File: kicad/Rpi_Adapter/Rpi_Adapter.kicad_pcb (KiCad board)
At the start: 2 copper layers, 65 x 22 mm, 49 parts, among them P1 CONN_02X20, P2 CONN_02X03

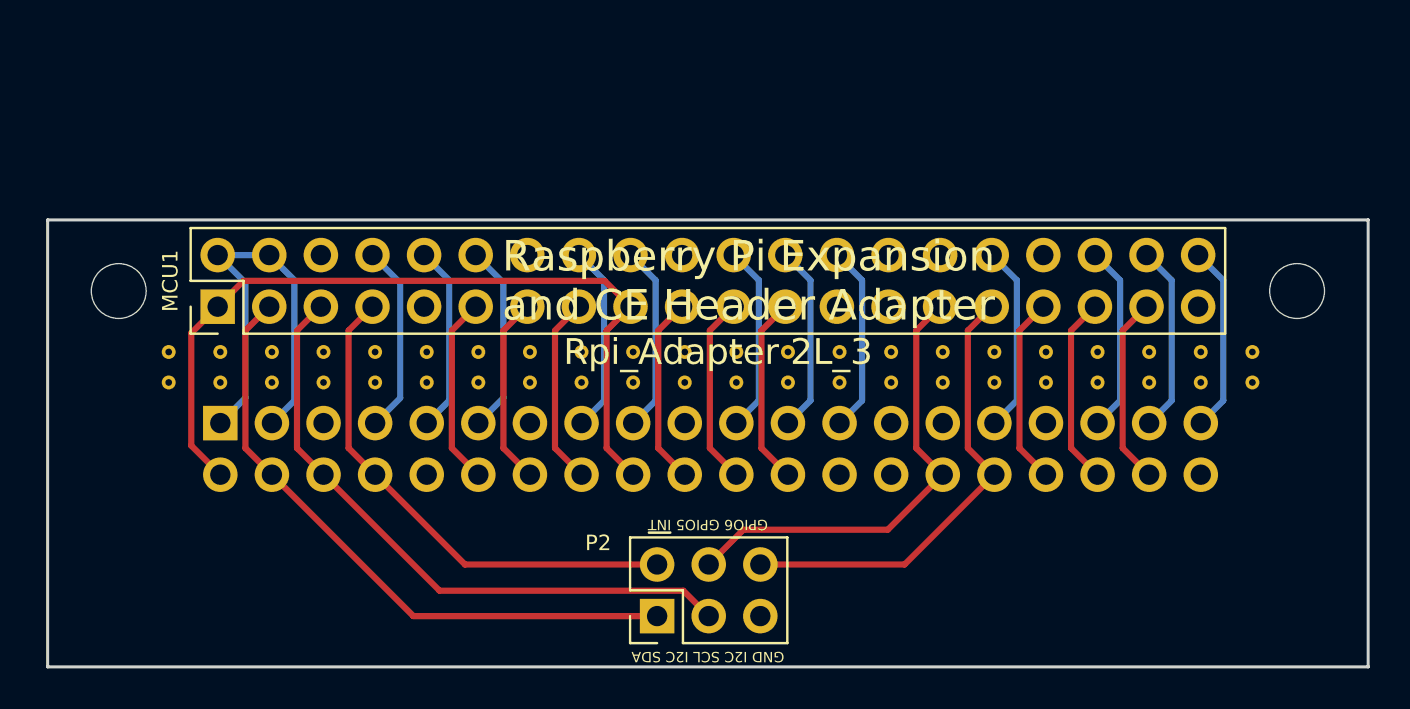
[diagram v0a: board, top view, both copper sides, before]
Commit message: Created the layout and submitted to OSH Park
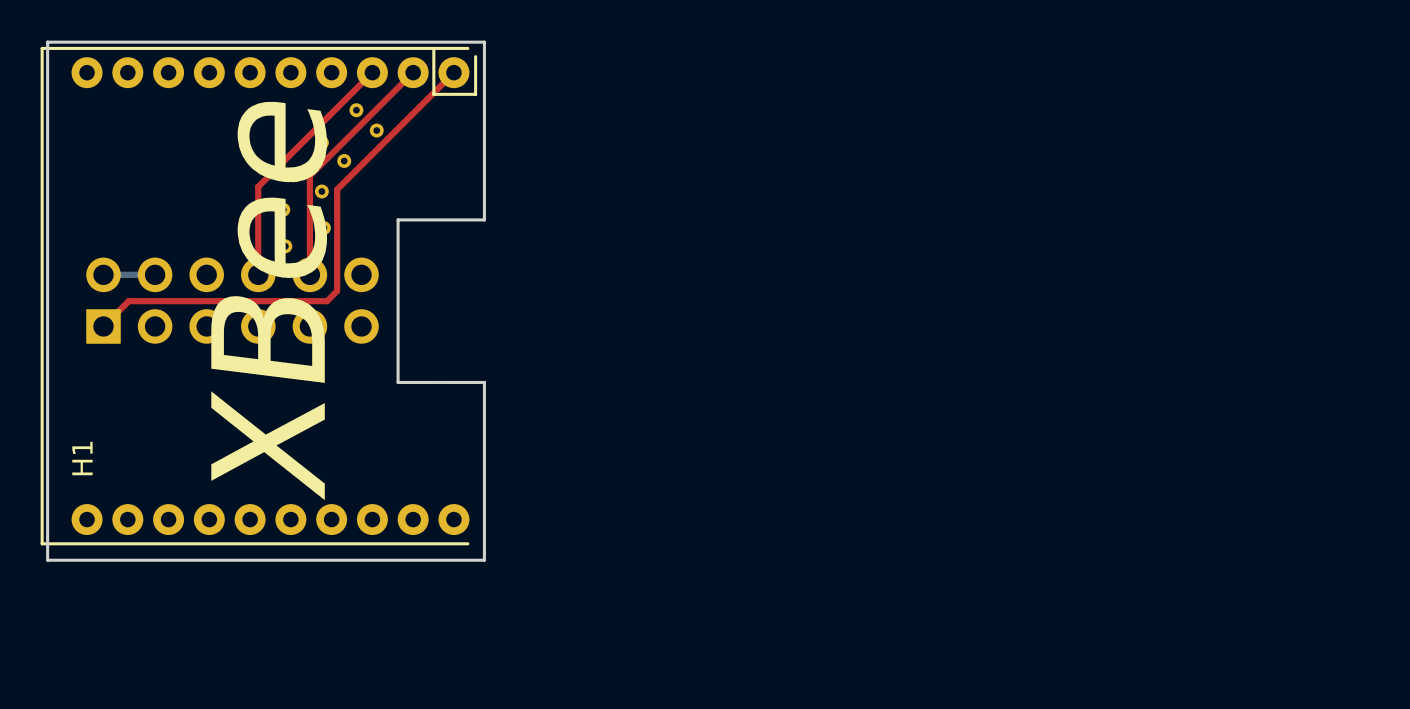
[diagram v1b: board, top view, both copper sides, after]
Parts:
- removed 1 (x2), 10, 11, 12, 13, 14, 15, 16, 17, 18, 19, 2, 20 (x2), 21 (x2), 22, 23, 24, 25, 26, 27, 28, 29, 3, 30, 31, 32, 33, 34, 35, 36, 37, 38, 39, 4, 40 (x2), 5, 6, 7, 8, 9: Stitch, Rpi_Adapter_Footprints:Stitch
- removed MCU1: RaspberryPi_3b, Rpi_Adapter_Footprints:Pin_Header_Straight_2x20_Pitch2.54mm
- removed MNT** (x2): MountingHole_2.7mm_M2.5, Mounting_Holes:MountingHole_2.7mm_M2.5
- removed P2: CONN_02X03, Pin_Headers:Pin_Header_Straight_2x03_Pitch2.54mm
- added ?: Stitch, Rpi_Adapter_Footprints:Stitch, F.Cu at (169.6, 42.4)
- added ?: Stitch, Rpi_Adapter_Footprints:Stitch, F.Cu at (167.6, 41.5)
- added ?: Stitch, Rpi_Adapter_Footprints:Stitch, F.Cu at (172.2, 37.6)
- added ?: Stitch, Rpi_Adapter_Footprints:Stitch, F.Cu at (169.5, 40.6)
- added ?: Stitch, Rpi_Adapter_Footprints:Stitch, F.Cu at (171.2, 36.6)
- added ?: Stitch, Rpi_Adapter_Footprints:Stitch, F.Cu at (170.6, 39.1)
- added ?: Stitch, Rpi_Adapter_Footprints:Stitch, F.Cu at (169.5, 38.2)
- added ?: Stitch, Rpi_Adapter_Footprints:Stitch, F.Cu at (168.1, 39.8)
- added ?: Stitch, Rpi_Adapter_Footprints:Stitch, F.Cu at (167.7, 43.3)
- added H1: DIGI_XBEE, Rpi_Adapter_Footprints:XBEE_S2C_Short, F.Cu at (176.0, 45.8)
- P1: value CONN_02X20 -> Raspberry PI; footprint Pin_Headers:Pin_Header_Straight_2x20_Pitch2.54mm -> Socket_Strips:Socket_Strip_Straight_2x06_Pitch2.54mm
- moved P1 7.46 mm to (158.8, 47.2)
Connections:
- P1 pad 1: /5V -> /3V3
- P1 pad 10: GND -> /UART0_Rx
- P1 pad 11: /GPIO_18 -> (no net)
- P1 pad 12: /GPIO_17 -> (no net)
- P1 pad 2: /3V3 -> /5V
- P1 pad 3: /5V -> (no net)
- P1 pad 4: /I2C1_SDA -> /5V
- P1 pad 5: GND -> (no net)
- P1 pad 6: /I2C1_SCL -> GND
- P1 pad 7: /UART0_Tx -> (no net)
- P1 pad 8: /GPIO_4 -> /UART0_Tx
- P1 pad 9: /UART0_Rx -> GND
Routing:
- net /I2C1_SCL: track 31.1 -> 0.00 mm
- net /I2C1_SDA: track 31.1 -> 0.00 mm
- net /GPIO_4: track 25.0 -> 0.00 mm
- net /GPIO_5: track 22.6 -> 0.00 mm
- net /GPIO_6: track 22.6 -> 0.00 mm
- net /5V: track 21.1 -> 2.54 mm
- net /3V3: track 40.1 -> 25.4 mm
- net /GPIO_18: track 9.35 -> 0.00 mm
- net /SPI0_SCLK: track 9.30 -> 0.00 mm
- net /SPI0_MISO: track 9.30 -> 0.00 mm
- net /GPIO_27: track 9.30 -> 0.00 mm
- net /GPIO_26: track 9.30 -> 0.00 mm
- net /GPIO_22: track 9.30 -> 0.00 mm
- net /GPIO_19: track 9.30 -> 0.00 mm
- net /SPI0_MOSI: track 9.30 -> 0.00 mm
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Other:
- board size 65 x 22 mm -> 21.5 x 25.5 mm
- board text removed: "GND I2C SCL I2C SDA"
- board text removed: "GPIO6 GPIO5 ~INT"
- board text removed: "Raspberry Pi Expansion and CE Header Adapter"
- board text removed: "Rpi_Adapter 2L_3"
